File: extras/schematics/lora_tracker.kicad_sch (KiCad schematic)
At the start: 27 parts, among them J1 ANT, J4 Conn_01x03_Female, SW1 SW_Push, SW2 EC11, U1 ESP32, U2 E22-400M30S, U3 RA-01, U4 INP441, U5 MAX98357A, U6 SSD1306

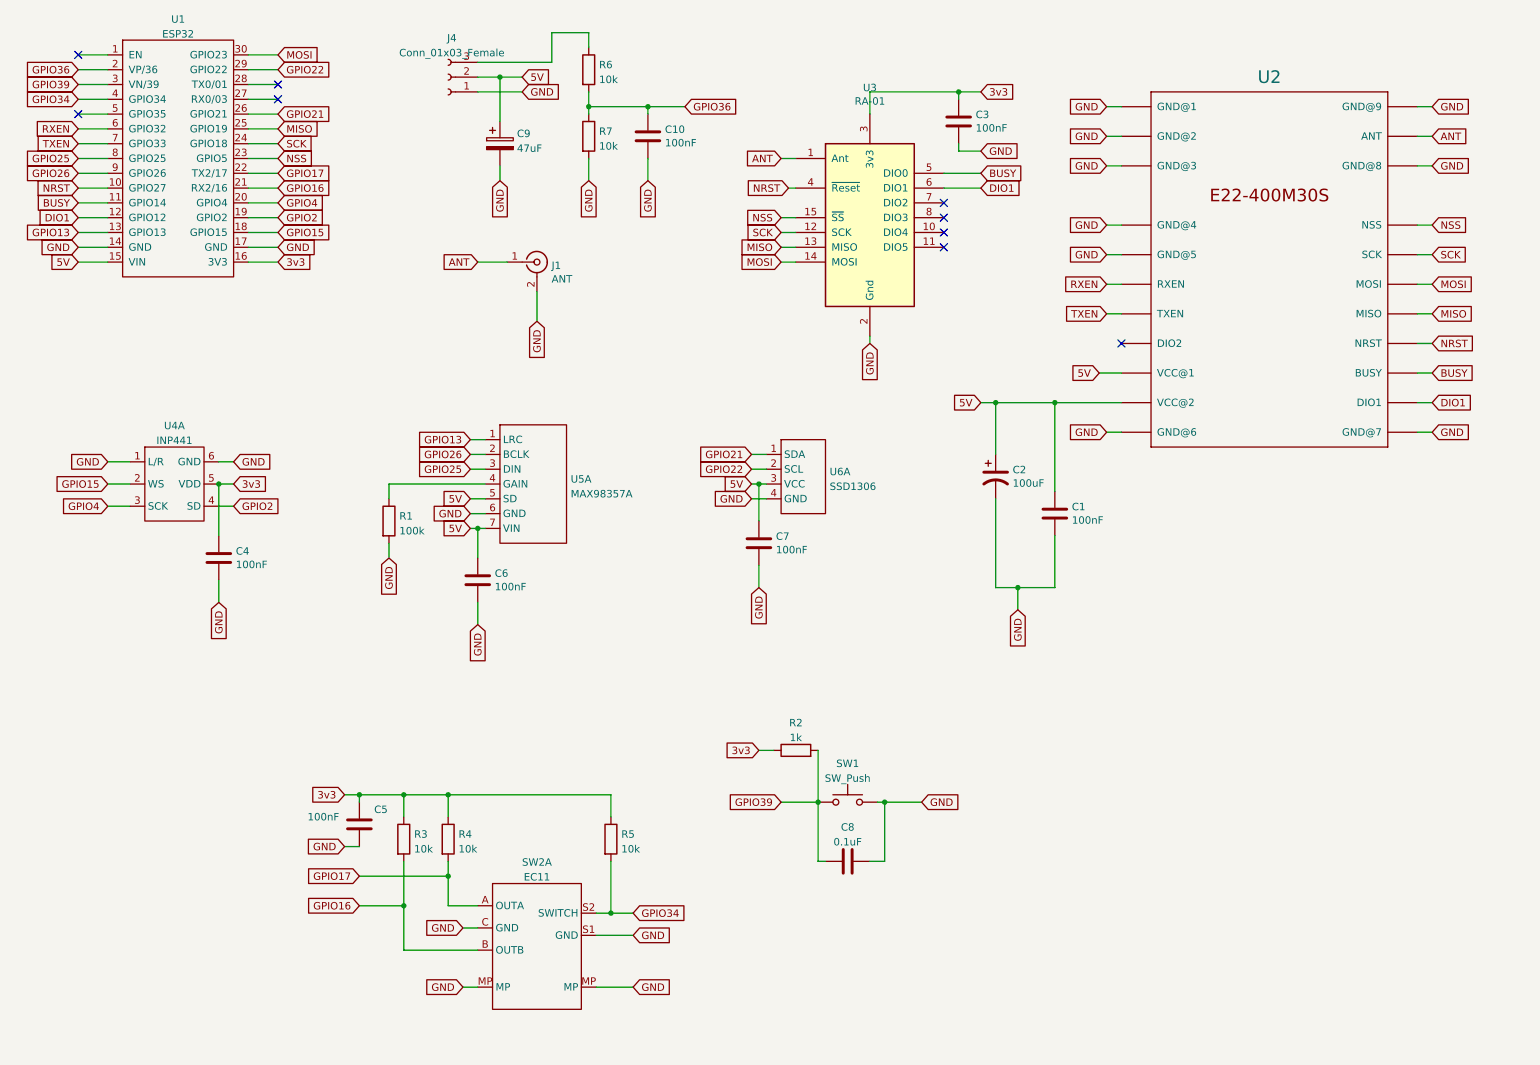
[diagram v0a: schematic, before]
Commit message: Update schematics
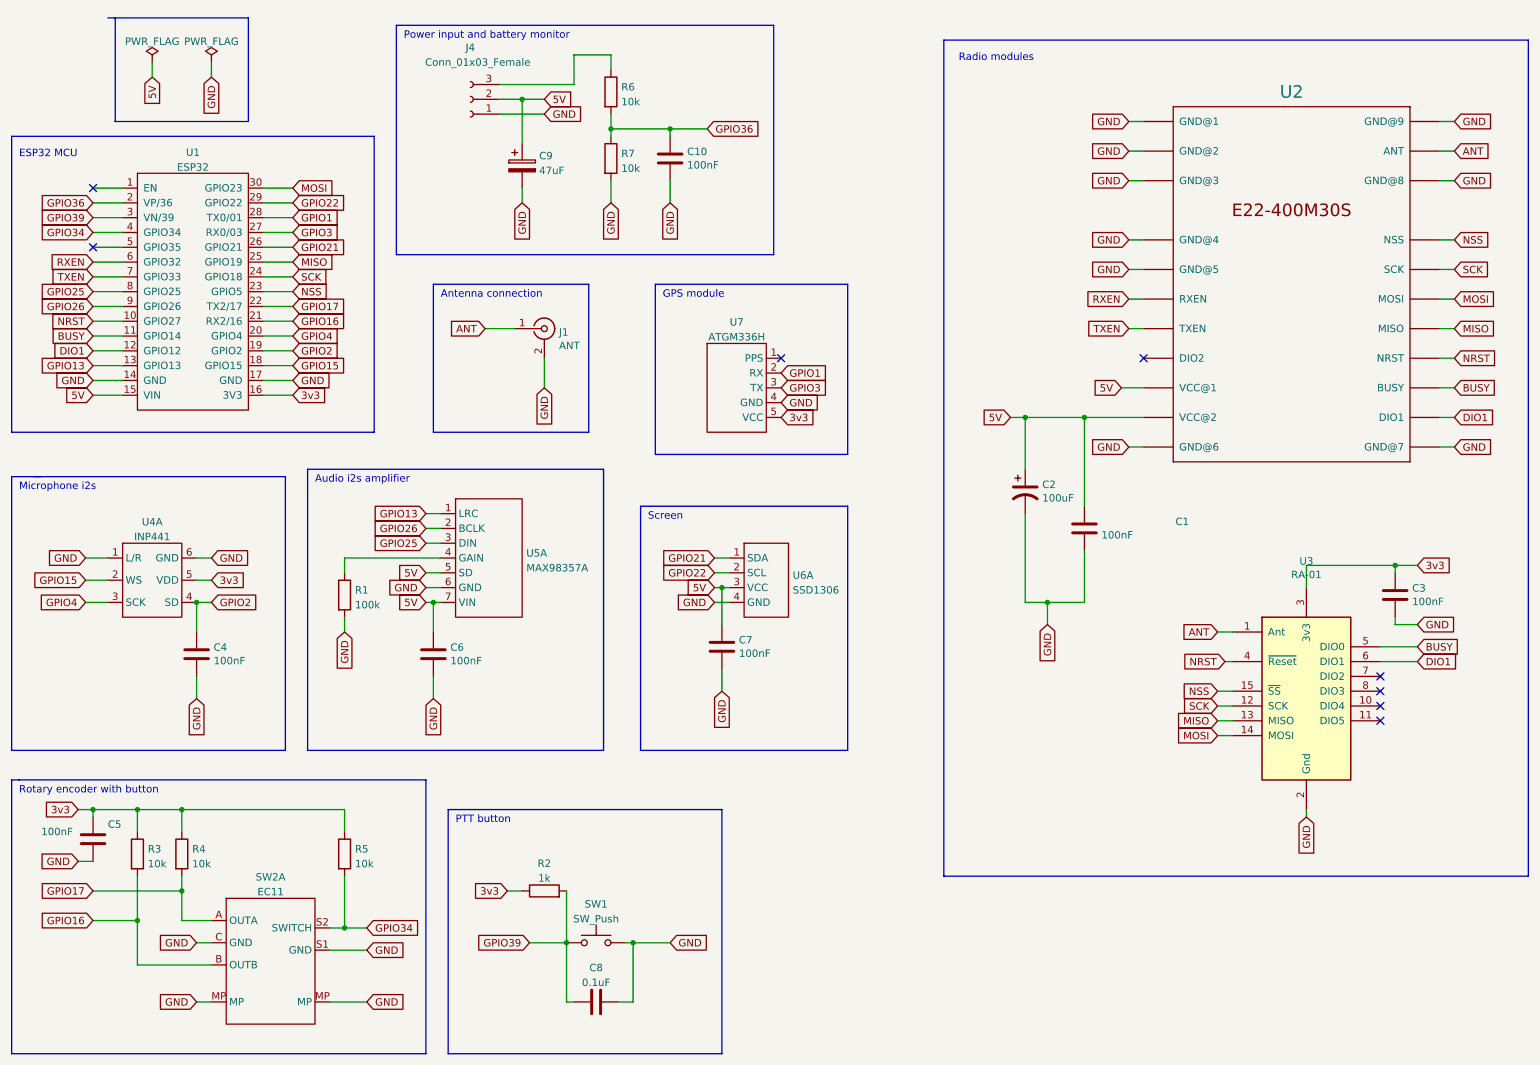
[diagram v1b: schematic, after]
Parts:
- added U7: ATGM336H, symbol lora_tracker:ATGM336H
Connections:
- net 3v3: now also U7.5 (VCC); no longer C4.1
- net GND: now also U7.4 (GND)
- net GPIO2: now also C4.1
- net GPIO3: now reaches U1.27 (RX0/03)
- net GPIO3: now also U7.3 (TX)
- net GPIO1: now reaches U1.28 (TX0/01)
- net GPIO1: now also U7.2 (RX)
- no-connect marks 9 -> 8
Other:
- note added: "Antenna connection"
- note added: "Audio i2s amplifier"
- note added: "ESP32 MCU"
- note added: "GPS module"
- note added: "Microphone i2s"
- note added: "PTT button"
- note added: "Power input and battery monitor"
- note added: "Radio modules"
- note added: "Rotary encoder with button"
- note added: "Screen"
- moved on the sheet: C1, C10, C2, C3, C4, C5, C6, C7, C8, C9, J1, J4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
